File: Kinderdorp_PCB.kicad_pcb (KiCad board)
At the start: 2 copper layers, 99.1 x 99.1 mm, 46 parts, among them Q1 2N7002_C306856, U1 AMS1117-3.3_C347222, U2 ESP32-C3-WROOM-02-N4(4MB)

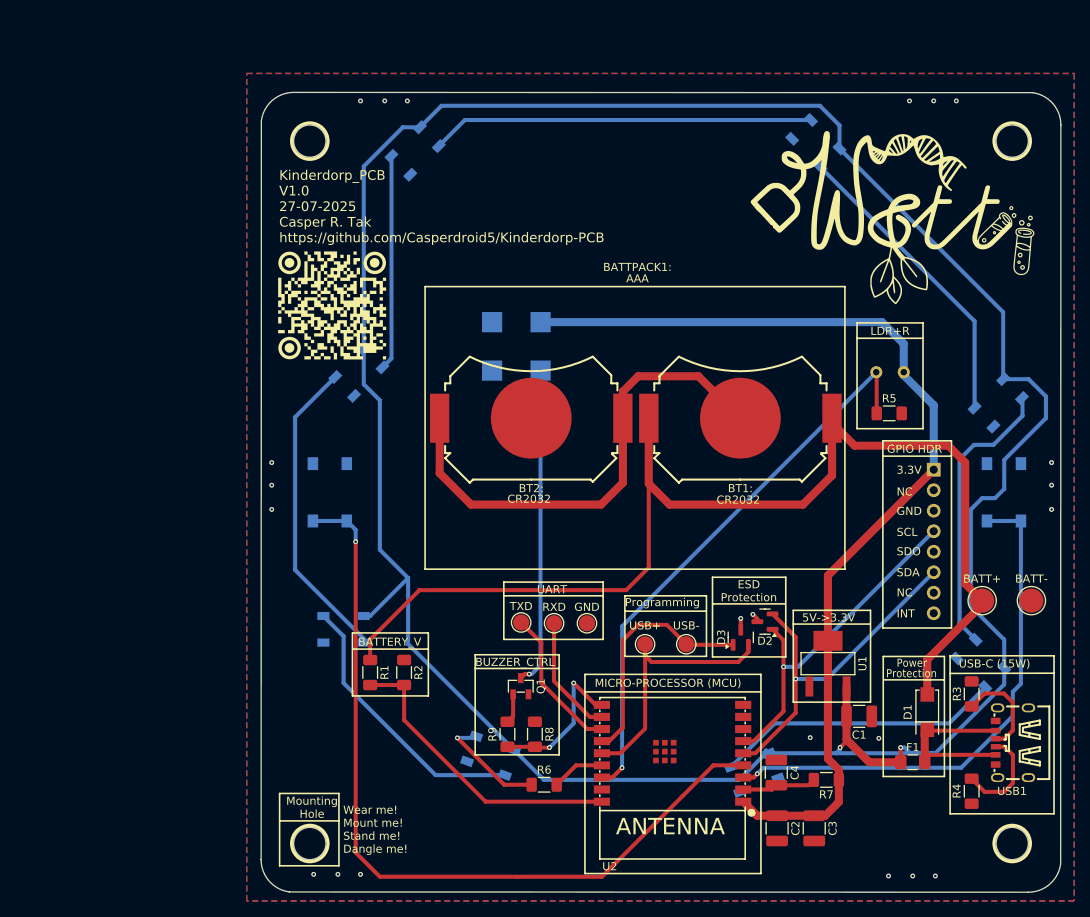
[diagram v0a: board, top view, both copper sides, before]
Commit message: moved board to centre
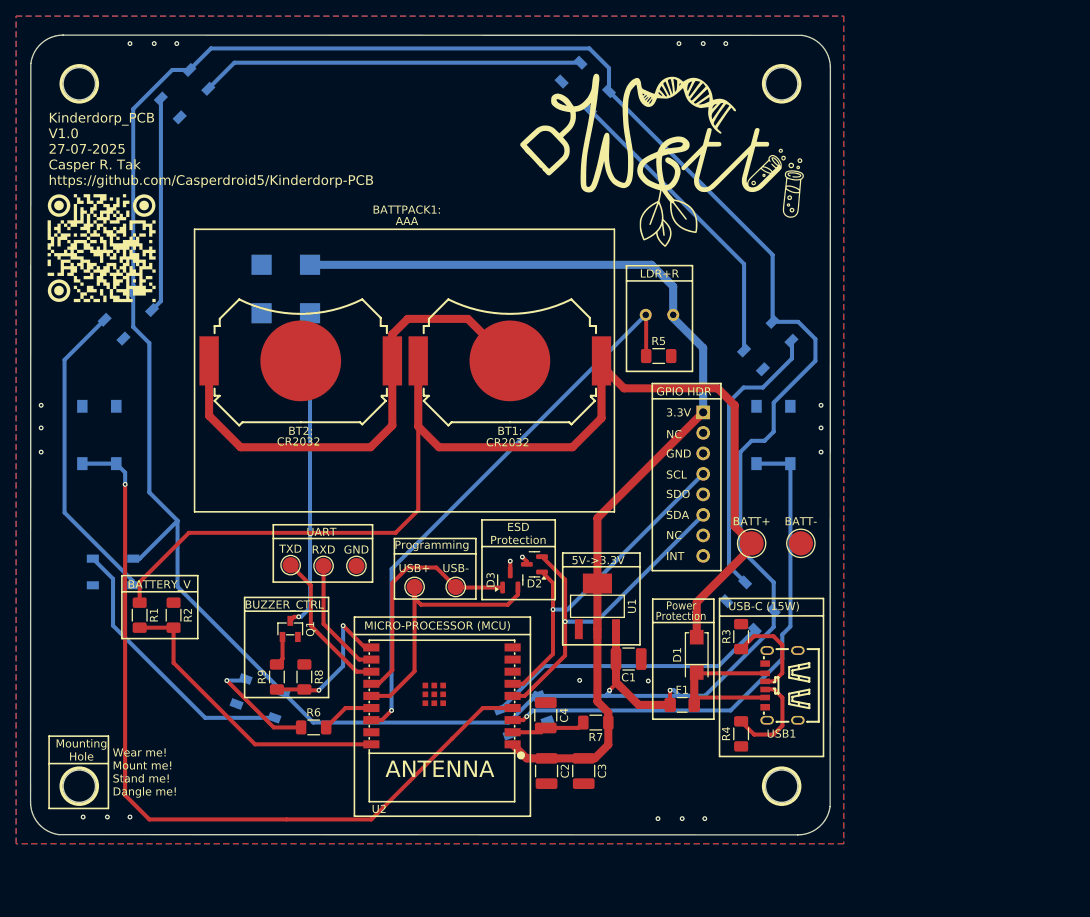
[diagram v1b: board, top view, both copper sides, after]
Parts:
- moved BT1: 29.4 mm to (150.1, 90.6)
- moved D1 29.4 mm to (173.2, 127.0)
- moved G*** 29.4 mm to (169.6, 64.8)
- moved LED5 29.4 mm to (159.4, 56.6)
- moved BUTTON1 29.4 mm to (182.7, 99.9)
- moved C1 29.4 mm to (164.8, 127.5)
- moved C3 29.4 mm to (159.2, 141.4)
- moved F1 29.4 mm to (171.4, 133.2)
- moved GND 29.4 mm to (131.1, 116.0)
- moved LED3 29.4 mm to (102.8, 84.9)
- moved LED4 29.4 mm to (109.8, 57.5)
- moved LED8 29.4 mm to (151.8, 134.5)
- moved LS1 29.4 mm to (122.3, 81.5)
- moved R1 29.4 mm to (104.2, 122.1)
- moved R3 29.4 mm to (178.7, 124.8)
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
